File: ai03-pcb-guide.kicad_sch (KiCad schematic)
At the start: 16 parts, among them J1 Conn_01x04_Socket, J2 AVR-ISP-6, U1 ATmega32U4-A, Y1 16MHz

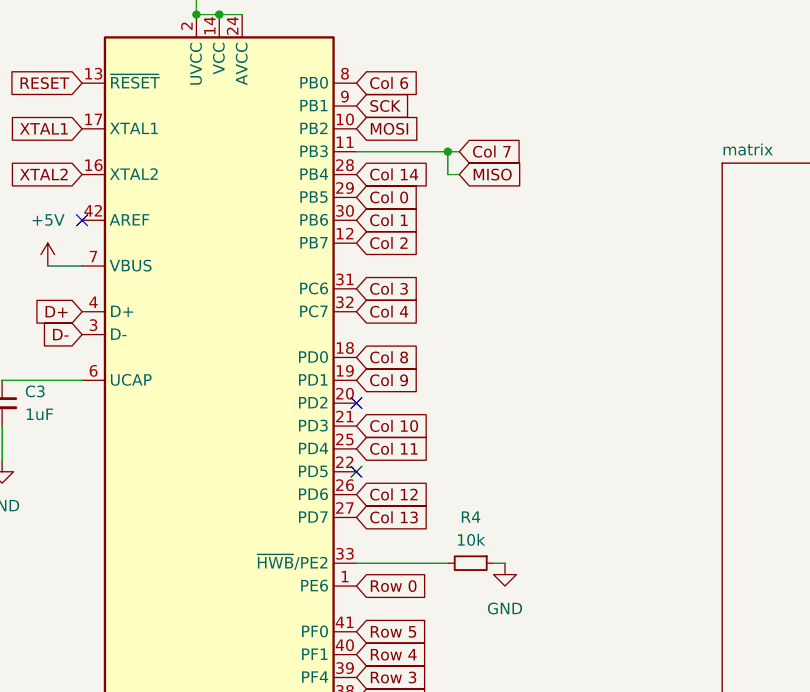
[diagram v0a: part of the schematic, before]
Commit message: more tracing work
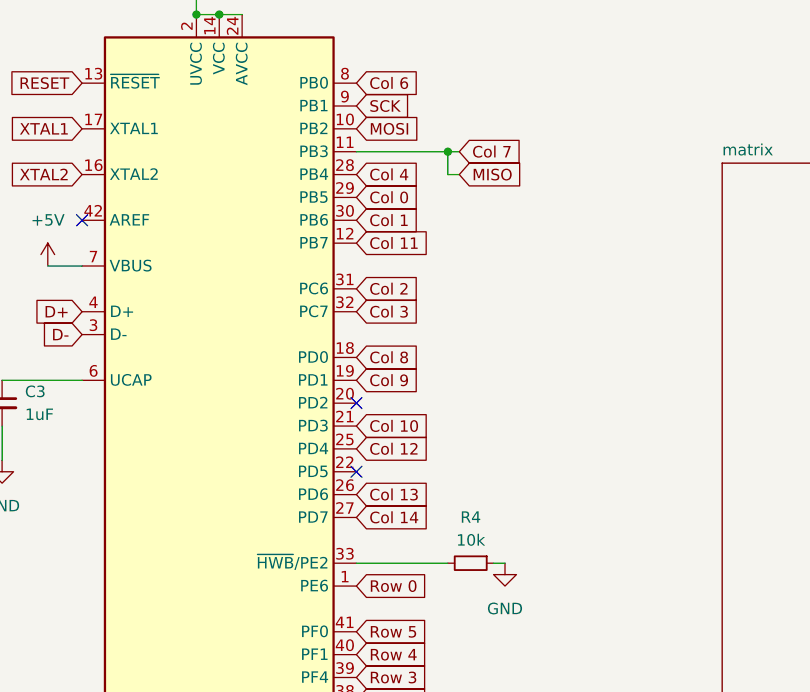
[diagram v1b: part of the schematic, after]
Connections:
- net Col 11: now also U1.12 (PB7); no longer U1.25 (PD4)
- net Col 12: now also U1.25 (PD4); no longer U1.26 (PD6)
- net Col 13: now also U1.26 (PD6); no longer U1.27 (PD7)
- net Col 14: now also U1.27 (PD7); no longer U1.28 (PB4)
- net Col 2: now also U1.31 (PC6); no longer U1.12 (PB7)
- net Col 3: now also U1.32 (PC7); no longer U1.31 (PC6)
- net Col 4: now also U1.28 (PB4); no longer U1.32 (PC7)

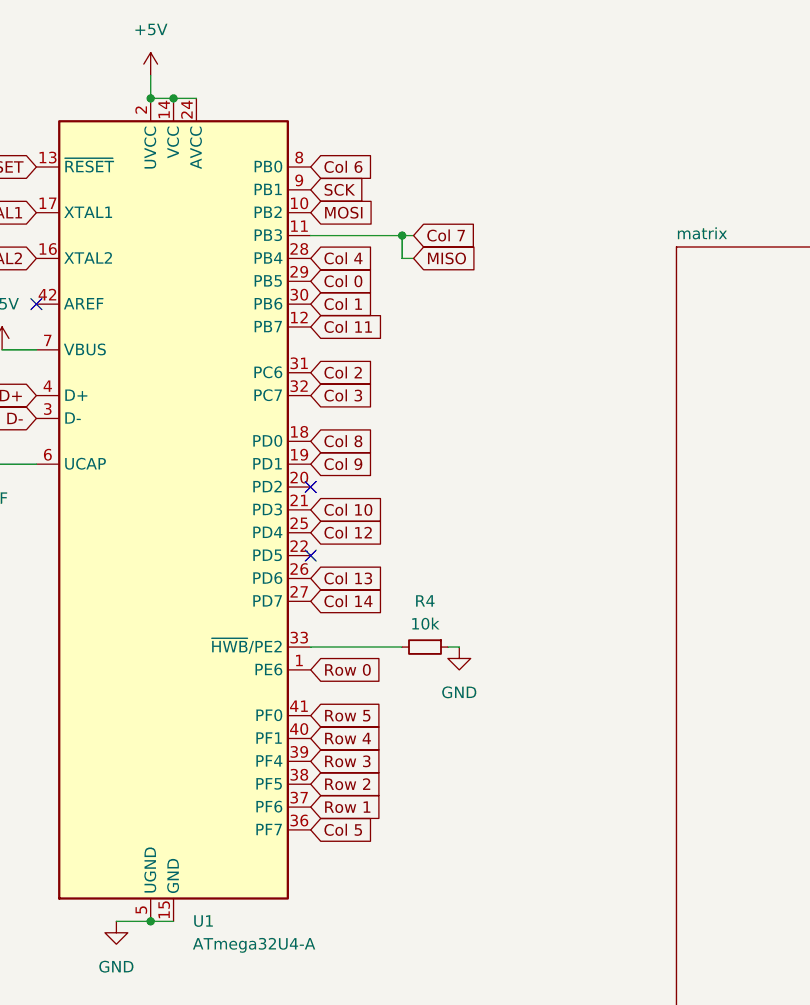
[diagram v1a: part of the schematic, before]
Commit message: most wiring complete
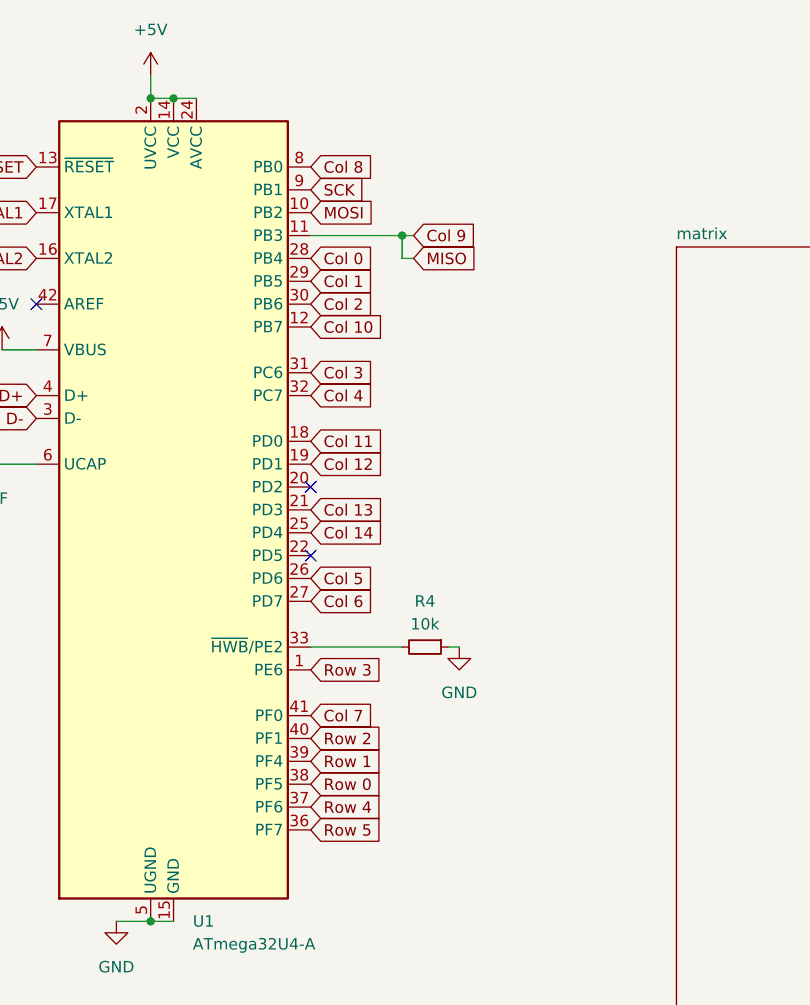
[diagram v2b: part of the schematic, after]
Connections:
- net Col 0: now also U1.28 (PB4); no longer U1.29 (PB5)
- net Col 1: now also U1.29 (PB5); no longer U1.30 (PB6)
- net Col 10: now also U1.12 (PB7); no longer U1.21 (PD3)
- net Col 11: now also U1.18 (PD0); no longer U1.12 (PB7)
- net Col 12: now also U1.19 (PD1); no longer U1.25 (PD4)
- net Col 13: now also U1.21 (PD3); no longer U1.26 (PD6)
- net Col 14: now also U1.25 (PD4); no longer U1.27 (PD7)
- net Col 2: now also U1.30 (PB6); no longer U1.31 (PC6)
- net Col 3: now also U1.31 (PC6); no longer U1.32 (PC7)
- net Col 4: now also U1.32 (PC7); no longer U1.28 (PB4)
- net Col 5: now also U1.26 (PD6); no longer U1.36 (PF7)
- net Col 6: now also U1.27 (PD7); no longer U1.8 (PB0)
- net Col 7: now also U1.41 (PF0); no longer J2.1 (MISO), U1.11 (PB3)
- net Col 8: now also U1.8 (PB0); no longer U1.18 (PD0)
- net Col 9: now also J2.1 (MISO), U1.11 (PB3); no longer U1.19 (PD1)
- net Row 0: now also U1.38 (PF5); no longer U1.1 (PE6)
- net Row 1: now also U1.39 (PF4); no longer U1.37 (PF6)
- net Row 2: now also U1.40 (PF1); no longer U1.38 (PF5)
- net Row 3: now also U1.1 (PE6); no longer U1.39 (PF4)
- net Row 4: now also U1.37 (PF6); no longer U1.40 (PF1)
- net Row 5: now also U1.36 (PF7); no longer U1.41 (PF0)
